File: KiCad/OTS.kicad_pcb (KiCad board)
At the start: 2 copper layers, 134.6 x 52.1 mm, 26 parts, among them P43 POWER_UP, U10 ProMini, U7 EZbluefruit, U8 LCD_TFT, U9 FeatherM0

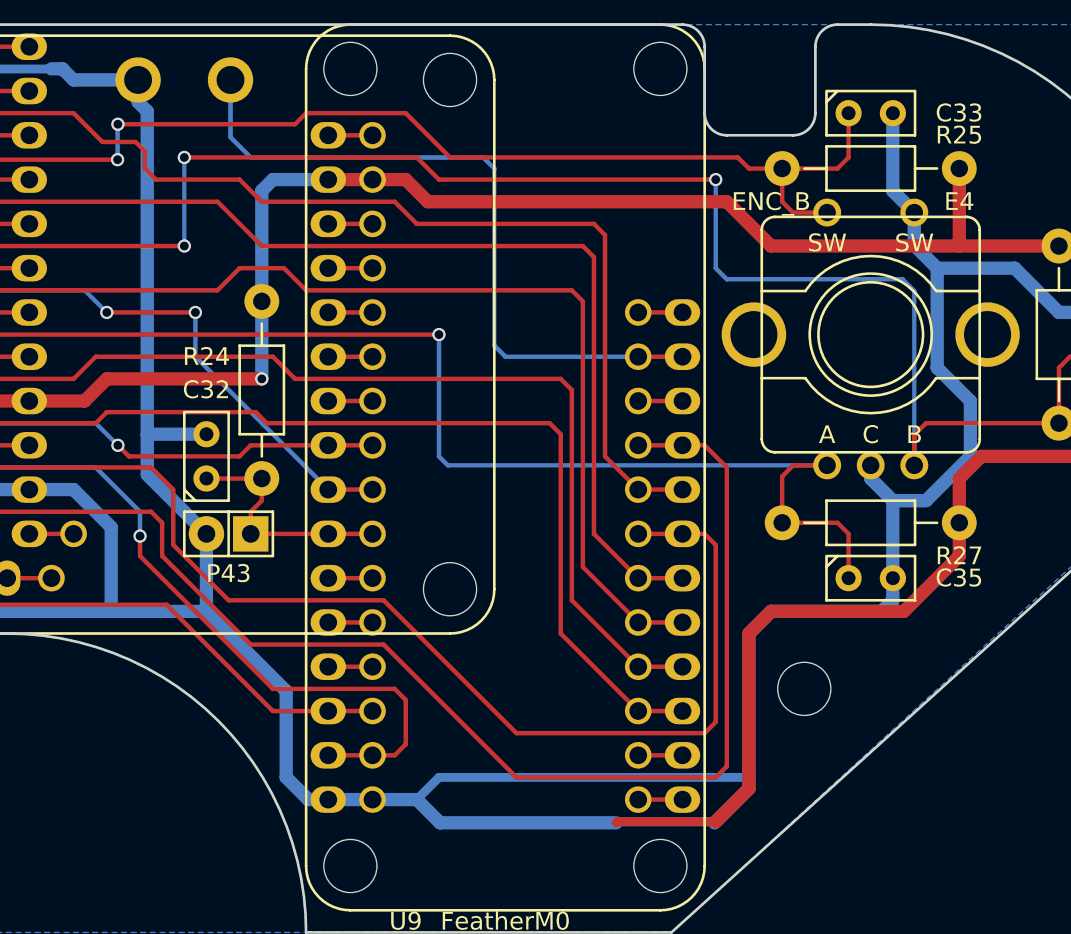
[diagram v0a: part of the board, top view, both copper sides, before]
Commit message: Git issue #1,#2,#5,#7 closed
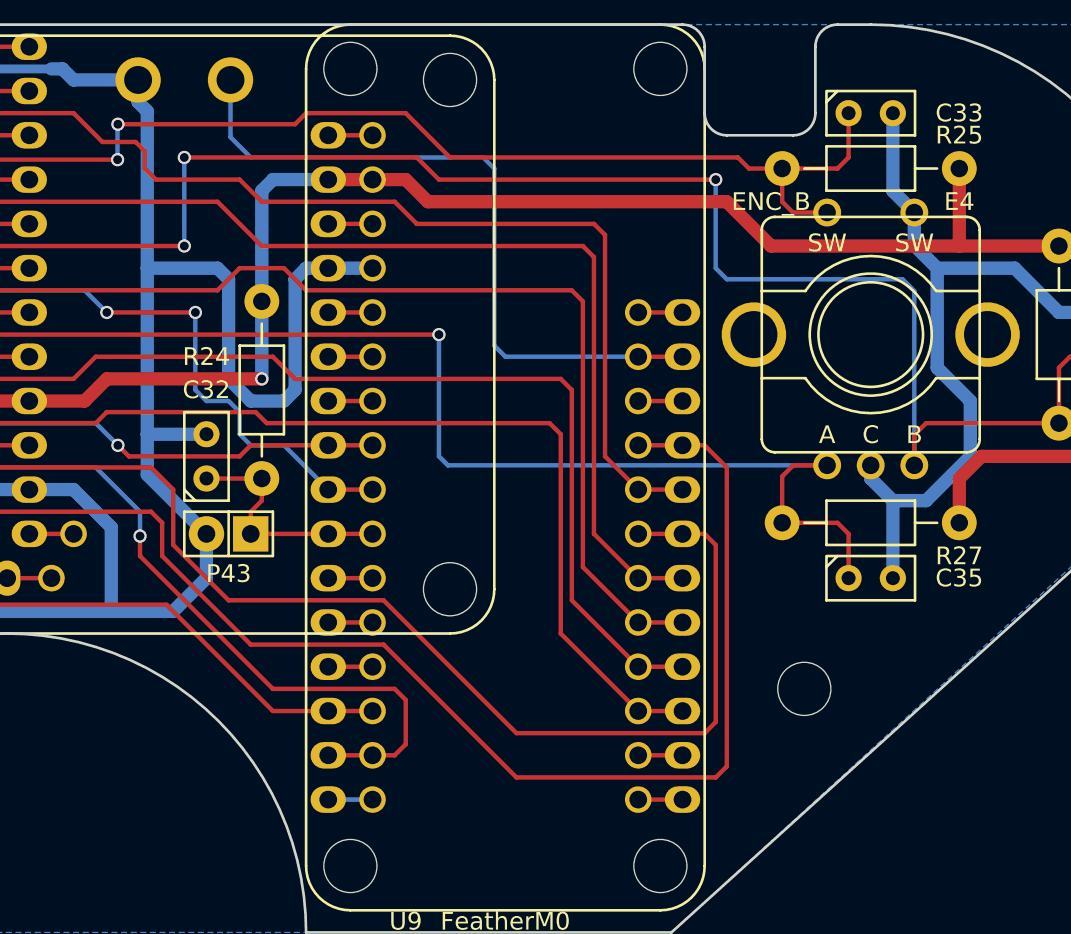
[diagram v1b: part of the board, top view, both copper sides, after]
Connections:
- U9 pad 16: Net-(U9-Pad16) -> /GND
- U9 pad 28: /GND -> Net-(U9-Pad28)
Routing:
- net /GND: track 376.1 -> 322.6 mm
- net /VCC: track 309.5 -> 267.8 mm
- net Net-(U9-Pad28): track 0.00 -> 2.54 mm
- net Net-(U9-Pad16): track 2.54 -> 0.00 mm
- net /L2: track 49.0 -> 50.9 mm
